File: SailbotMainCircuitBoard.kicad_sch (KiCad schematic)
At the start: 0 parts

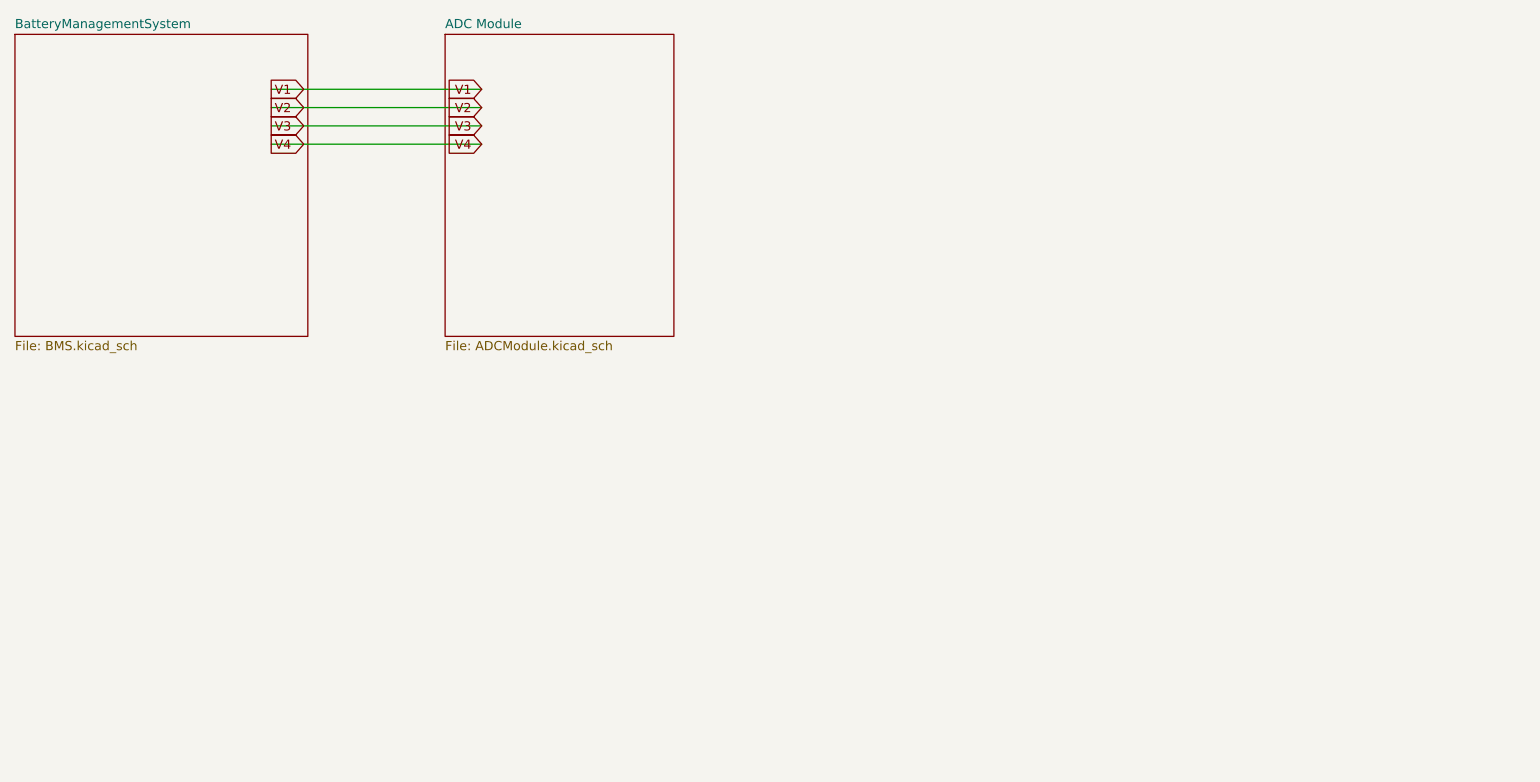
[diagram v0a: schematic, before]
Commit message: Pushing updated schematics
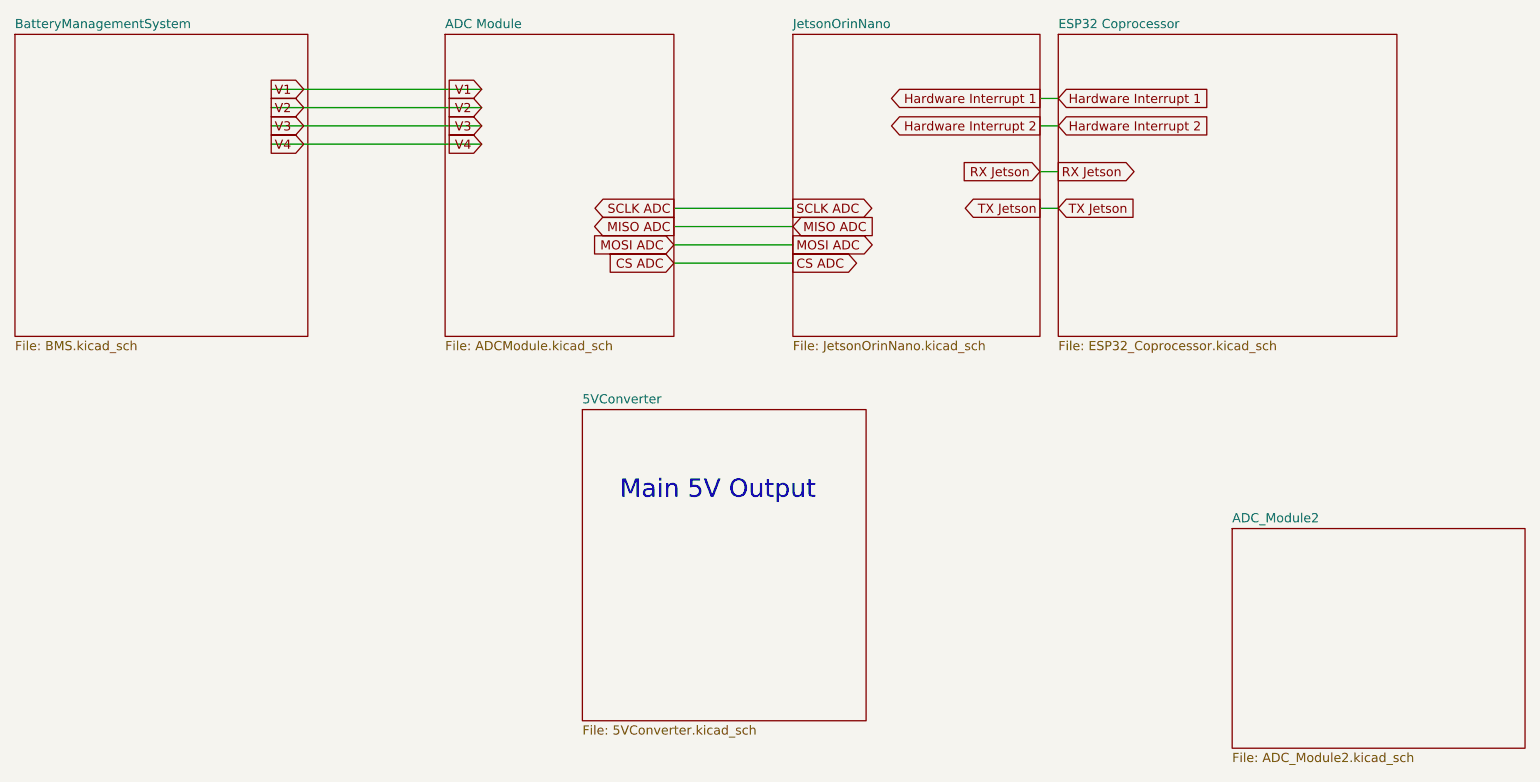
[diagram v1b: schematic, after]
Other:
- added sheet 5VConverter (5VConverter.kicad_sch)
- added sheet ADC_Module2 (ADC_Module2.kicad_sch)
- added sheet ESP32 Coprocessor (ESP32_Coprocessor.kicad_sch)
- added sheet JetsonOrinNano (JetsonOrinNano.kicad_sch)
- note added: "Main 5V Output"
